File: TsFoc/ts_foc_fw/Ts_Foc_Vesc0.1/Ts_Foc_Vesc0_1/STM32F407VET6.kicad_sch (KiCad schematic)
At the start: 26 parts, among them SW2 BOTTOM, U3 STM32F407VET6, X1 25Mhz

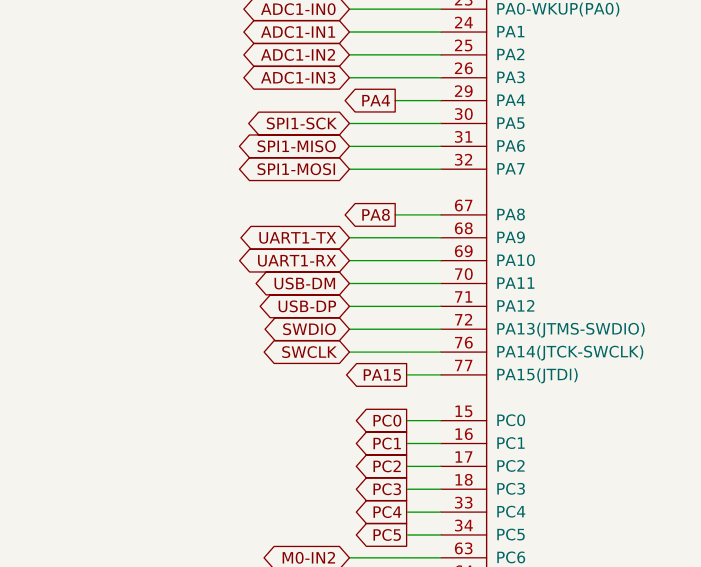
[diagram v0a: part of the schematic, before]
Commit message: 电源走线完成
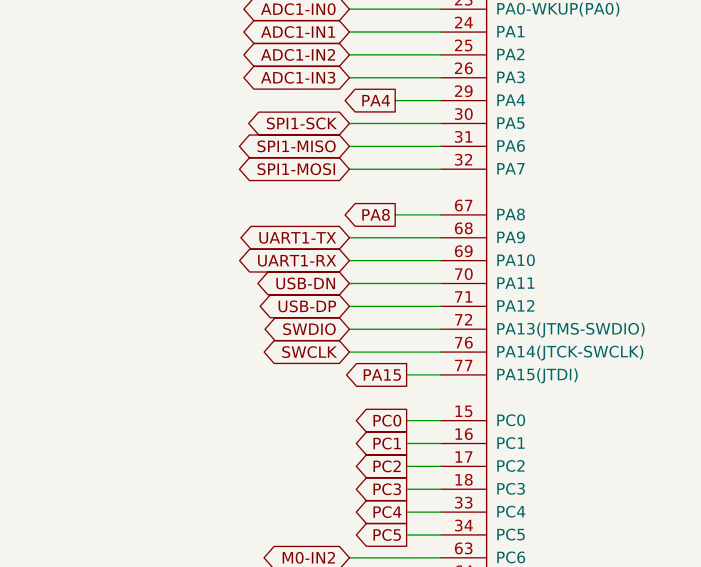
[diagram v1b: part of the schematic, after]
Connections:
- net USB-DM renamed USB-DN
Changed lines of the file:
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@@
 		)
 	)
-	(global_label "USB-DM"
+	(global_label "USB-DN"
 		(shape bidirectional)
 		(at 48.26 54.61 180)
@@
 		)
 		(property "Intersheetrefs" "${INTERSHEET_REFS}"
-			(at 36.0597 54.61 0)
+			(at 36.1806 54.61 0)
 			(effects
 				(font
